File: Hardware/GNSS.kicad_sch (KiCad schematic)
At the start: 26 parts, among them J1 U.FL_SMD, Q3 BSS138, U13 74HC4052D, U2 mosaic-X5

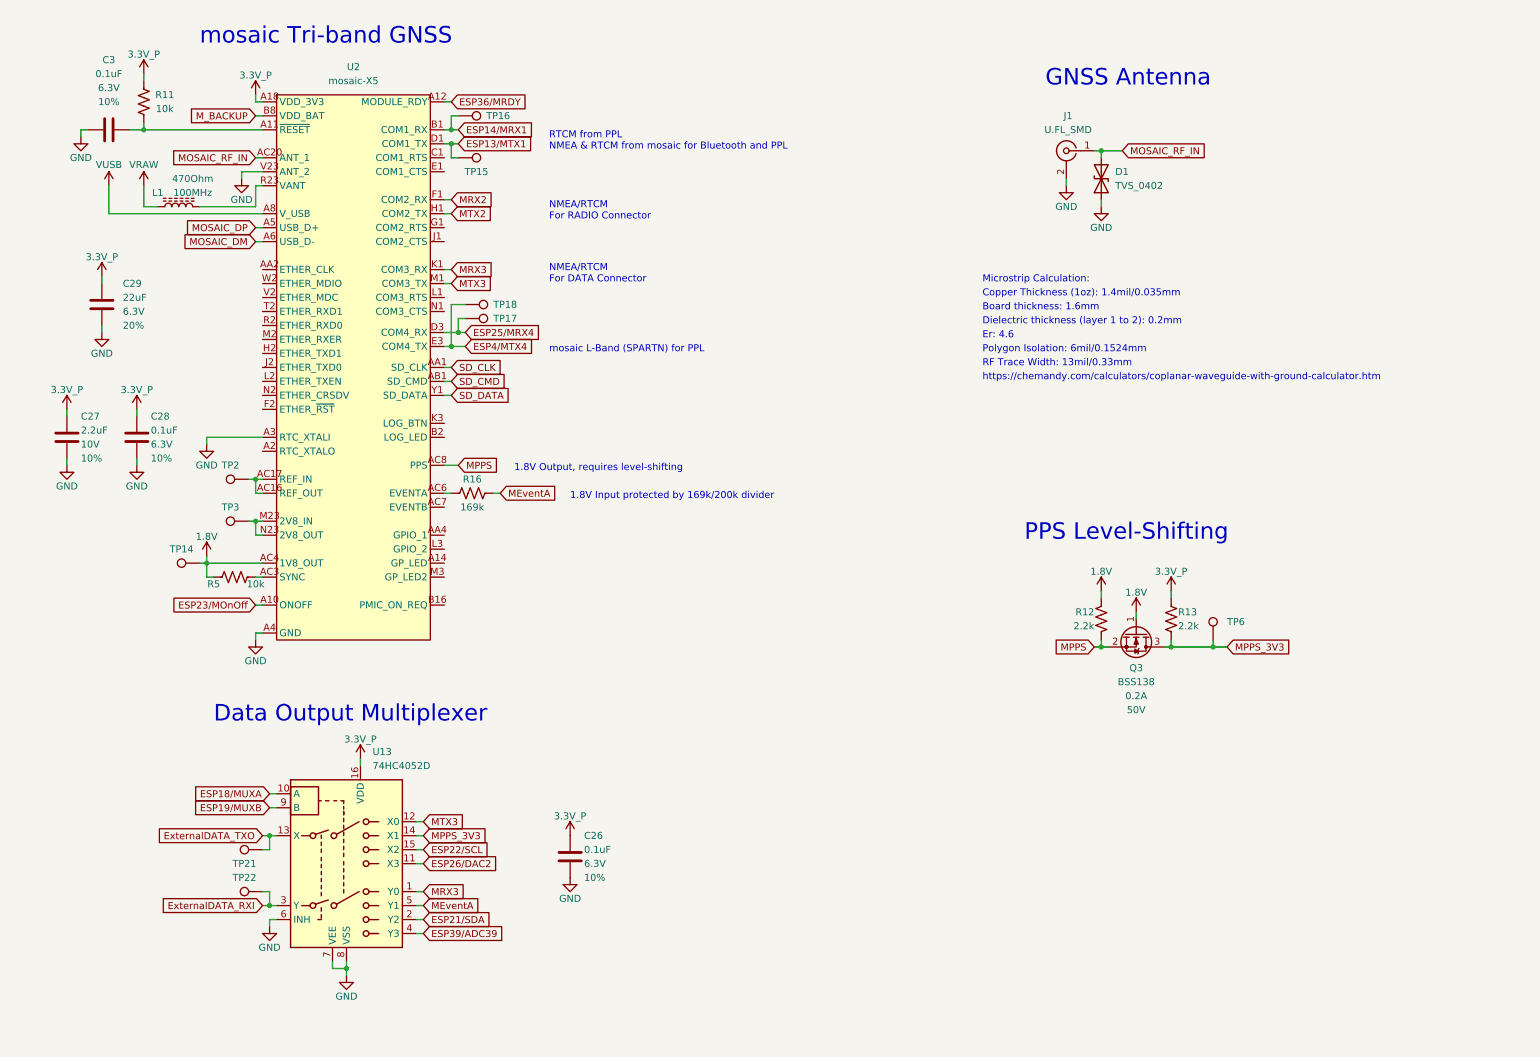
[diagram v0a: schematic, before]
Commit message: v1.1 routed
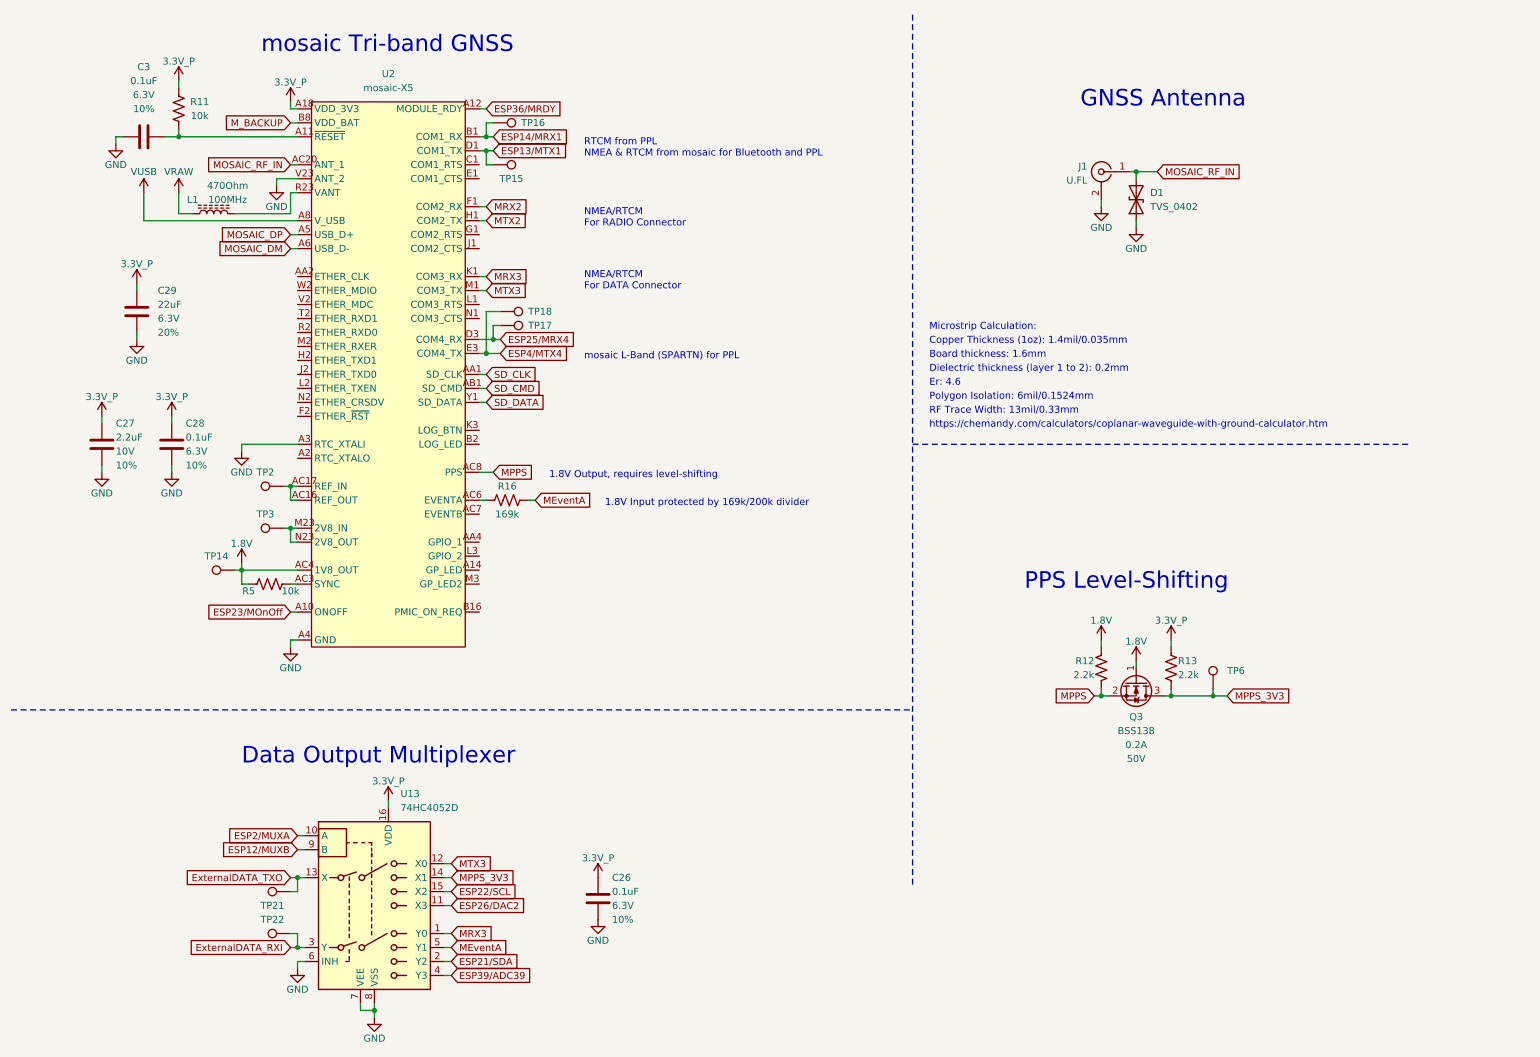
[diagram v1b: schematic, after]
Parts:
- removed J1: U.FL_SMD, SparkFun-Connector:U.FL, symbol SparkFun-RF:U.FL_SMD
- added J1: U.FL, SparkFun-Connector:U.FL, symbol SparkFun-RF:U.FL
- TP21, TP22, TP6: footprint SparkFun-Connector:1X01 -> SparkFun-Connector:1x01
- U13: footprint SparkFun-Semiconductor-Standard:SO16 -> SparkFun-Semiconductor-Standard:SO-16
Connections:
- net GND: now also J1.2 (Ext)
- net MOSAIC_RF_IN: now also J1.1 (In)
- net ESP18/MUXA renamed ESP2/MUXA
- net ESP19/MUXB renamed ESP12/MUXB
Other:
- moved on the sheet: C26, C27, C28, C29, C3, D1, L1, Q3, R11, R12, R13, R16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

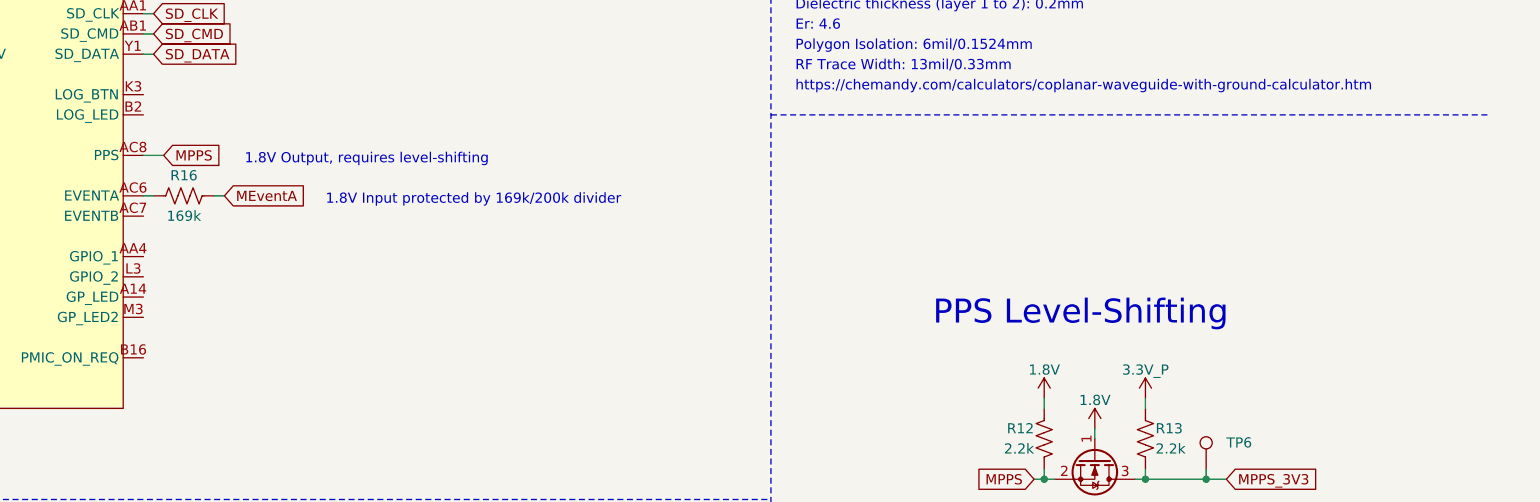
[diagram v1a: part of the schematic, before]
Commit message: V1.1 Panelized
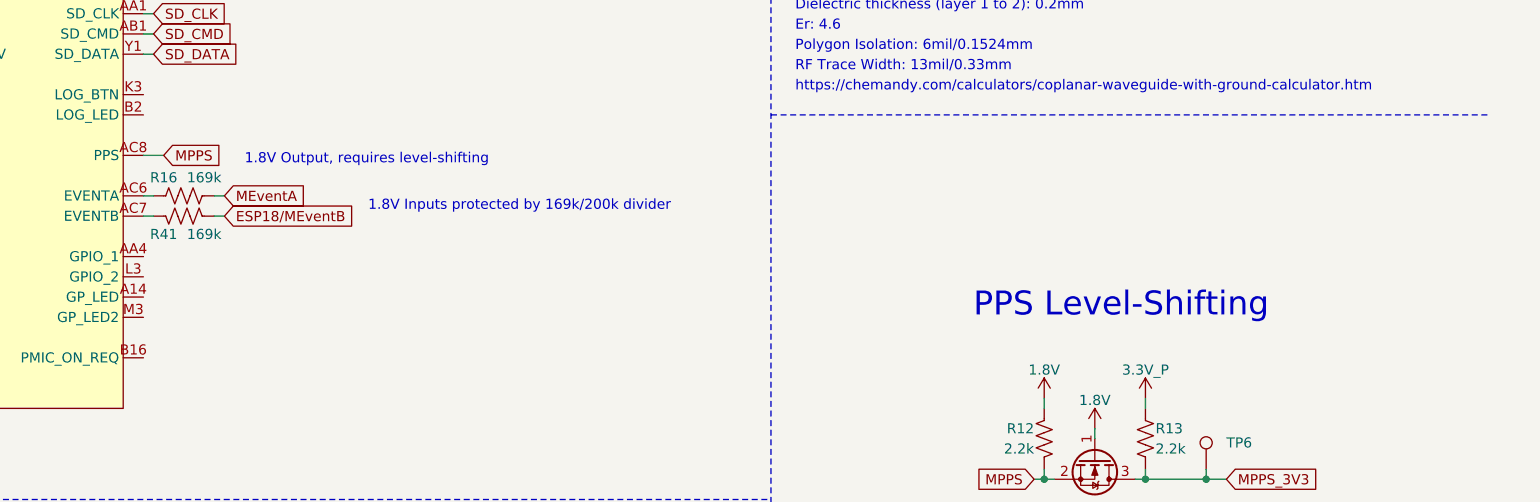
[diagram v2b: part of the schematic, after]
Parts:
- added R41: 169k, SparkFun-Resistor:R_0603_1608Metric, symbol SparkFun-Resistor:169k_0603
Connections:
- net at U2.AC7 (EVENTB): now also R41.2
- new net ESP18/MEventB: R41.1
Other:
- note added: "1.8V Inputs protected by 169k/200k divider"
- note removed: "1.8V Input protected by 169k/200k divider"
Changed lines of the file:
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@@
 	(wire
 		(pts
+			(xy 106.68 104.14) (xy 107.95 104.14)
+		)
+		(stroke
+			(width 0)
+			(type default)
+		)
+	)
+	(wire
+		(pts
 			(xy 210.82 137.16) (xy 212.09 137.16)
 		)
@@
 	(wire
 		(pts
+			(xy 97.79 104.14) (xy 99.06 104.14)
+		)
+		(stroke
+			(width 0)
+			(type default)
+		)
+	)
+	(wire
+		(pts
 			(xy 63.5 106.68) (xy 63.5 109.22)
 		)
@@
 	(text "PPS Level-Shifting\n"
 		(exclude_from_sim no)
-		(at 196.85 118.11 0)
+		(at 201.93 117.094 0)
 		(effects
 			(font
@@
 		)
 	)
-	(text "1.8V Input protected by 169k/200k divider"
+	(text "1.8V Inputs protected by 169k/200k divider"
 		(exclude_from_sim no)
-		(at 120.65 102.87 0)
+		(at 125.984 103.632 0)
 		(effects
 			(font
@@
 		)
 	)
+	(global_label "ESP18{slash}MEventB"
+		(shape input)
+		(at 107.95 104.14 0)
+		(fields_autoplaced yes)
+		(effects
+			(font
+				(size 1.27 1.27)
+			)
+			(justify left)
+		)
+		(property "Intersheetrefs" "${INTERSHEET_REFS}"
+			(at 124.6631 104.14 0)
+			(effects
+				(font
+					(size 1.27 1.27)
+				)
+				(justify left)
+				(hide yes)
+			)
+		)
+	)
 	(global_label "ExternalDATA_TXO"
 		(shape input)
@@
 		(dnp no)
 		(property "Reference" "R16"
-			(at 102.87 99.06 0)
+			(at 100.33 99.314 0)
 			(effects
 				(font
@@
 		)
 		(property "Value" "169k"
-			(at 102.87 104.14 0)
+			(at 105.41 99.314 0)
 			(effects
 				(font
@@
 					(unit 1)
 				)
+			)
+		)
+	)
+	(symbol
+		(lib_id "SparkFun-Resistor:169k_0603")
+		(at 102.87 104.14 0)
+		(mirror x)
+		(unit 1)
+		(exclude_from_sim no)
+		(in_bom yes)
+		(on_board yes)
+		(dnp no)
+		(property "Reference" "R41"
+			(at 100.33 106.426 0)
+			(effects
+				(font
+					(size 1.27 1.27)
+				)
+			)
+		)
+		(property "Value" "169k"
+			(at 105.41 106.426 0)
+			(effects
+				(font
+					(size 1.27 1.27)
+				)
+			)
+		)
+		(property "Footprint" "SparkFun-Resistor:R_0603_1608Metric"
+			(at 102.87 99.822 0)
+			(effects
+				(font
+					(size 1.27 1.27)
+				)
+				(hide yes)
+			)
+		)
+		(property "Datasheet" "https://www.vishay.com/docs/20035/dcrcwe3.pdf"
+			(at 102.87 95.25 0)
+			(effects
+				(font
+					(size 1.27 1.27)
+				)
+				(hide yes)
+			)
+		)
+		(property "Description" "Resistor"
+			(at 102.87 104.14 0)
+			(effects
+				(font
+					(size 1.27 1.27)
+				)
+				(hide yes)
+			)
+		)
+		(property "PROD_ID" "RES-14394"
+			(at 102.87 97.79 0)
+			(effects
+				(font
+					(size 1.27 1.27)
+				)
+				(hide yes)
+			)
+		)
+		(pin "1"
+		)
+		(pin "2"
+		)
+		(instances
+			(project "SparkFun_RTK_Facet_mosaic"
+				(path "/e3dd3ae4-244d-4cba-9cca-5d2abf83f29a/1004b21d-c362-4c5d-adad-4952c3ff3811"
+					(reference "R41")
+					(unit 1)
+				)
